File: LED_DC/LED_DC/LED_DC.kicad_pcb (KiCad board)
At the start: 2 copper layers, 98.4 x 98.4 mm, 49 parts, among them J1 Conn_01x04, J2 Display Port GPIO, J3 Conn_01x05, Q1 FDV304P, Q2 FDV304P, Q3 FDV304P, Q4 FDV304P, Q5 FDV304P, Q6 FDV304P, Q7 FDV304P, Q8 FDV304P, SW1 SW_Push_45deg, SW2 SW_Push_45deg, SW3 SW_Push_45deg, SW4 SW_Push_45deg, U1 74HC238, U2 ULN2803A, U3 KCSA02-136, U4 KCSA02-136, U5 KCSA02-136, U6 KCSA02-136, U7 KCSA02-136, U8 KCSA02-136, U9 KCSA02-136

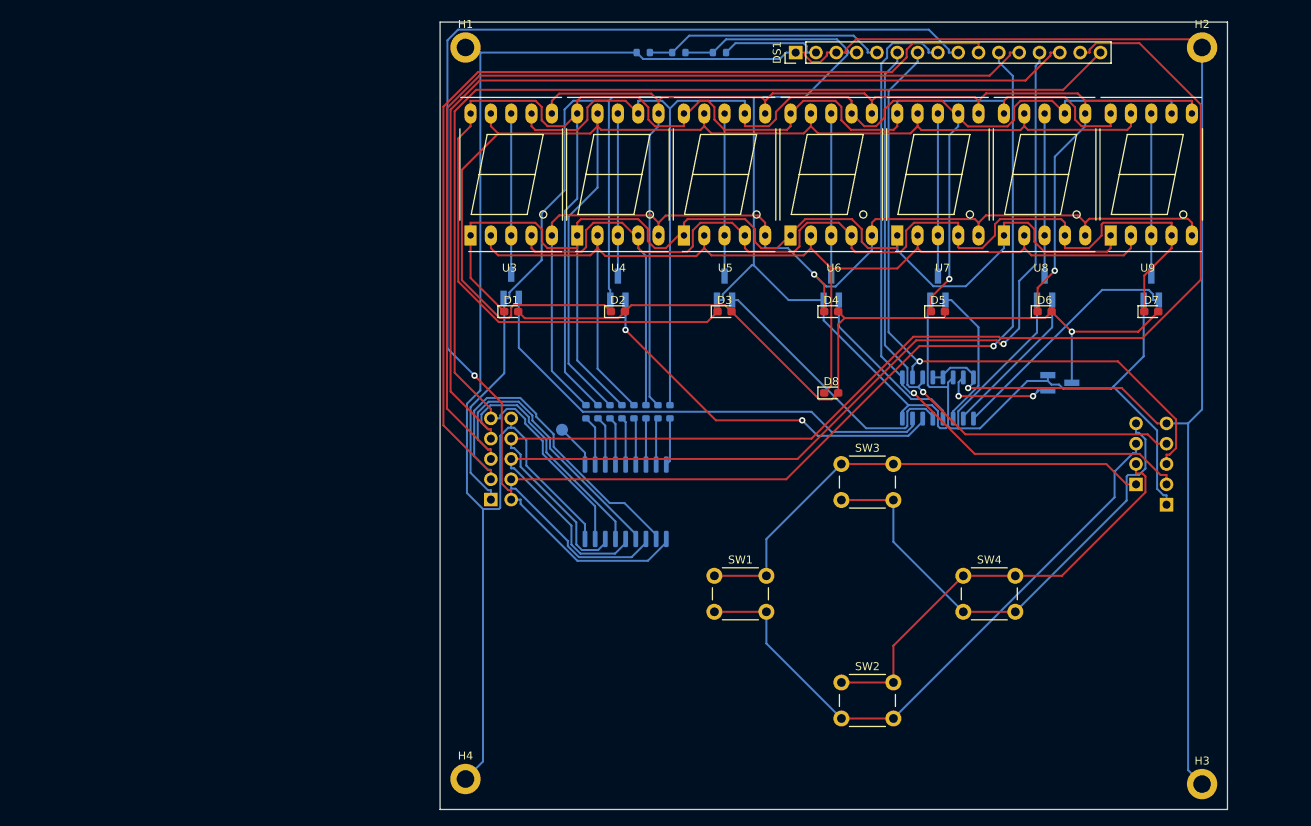
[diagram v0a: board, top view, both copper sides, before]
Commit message: Updated PCB.
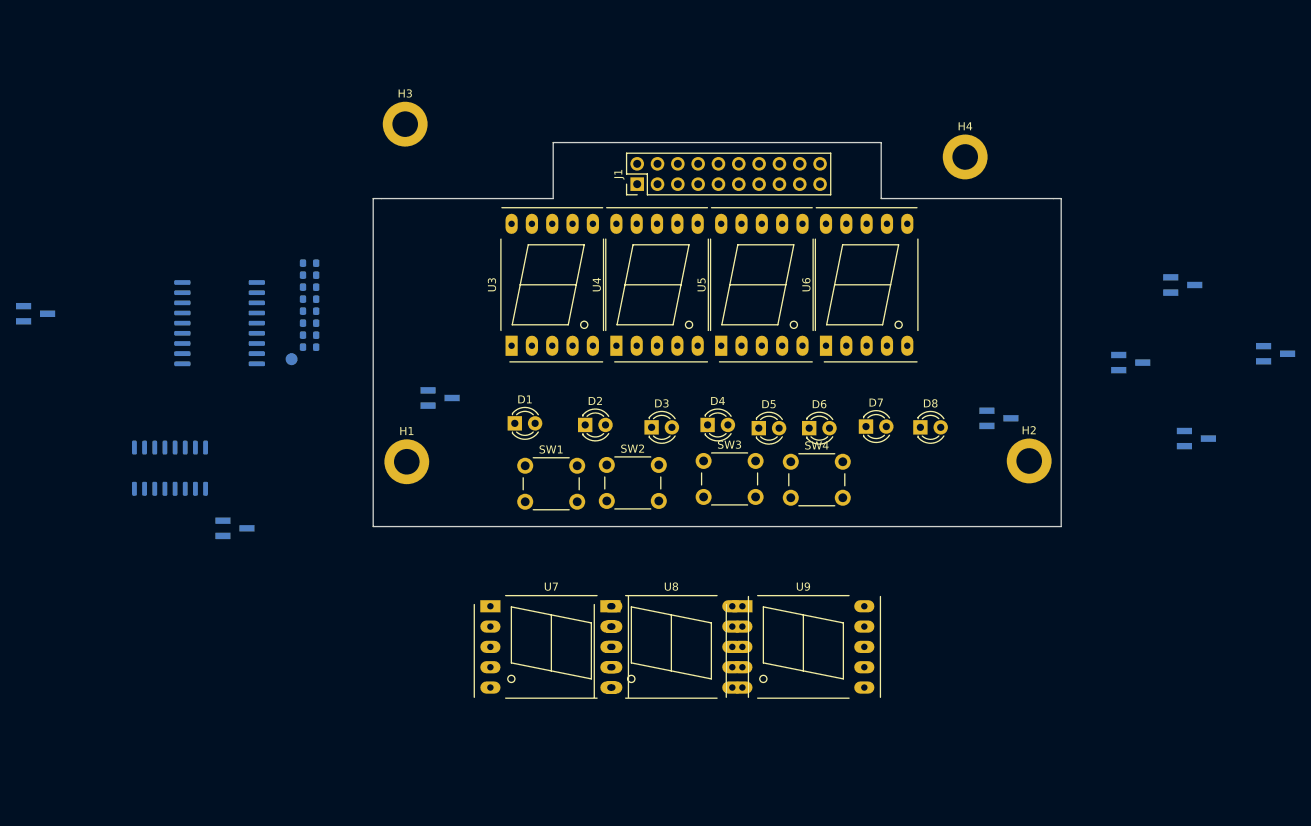
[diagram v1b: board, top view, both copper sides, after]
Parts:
- removed DS1: HY1602E, Connector_PinHeader_2.54mm:PinHeader_1x16_P2.54mm_Vertical
- removed J2: Display Port GPIO, Connector_PinHeader_2.54mm:PinHeader_2x05_P2.54mm_Vertical
- removed J3: Conn_01x05, Connector_PinHeader_2.54mm:PinHeader_1x05_P2.54mm_Vertical
- removed R1, R2, R3: R_Small, Resistor_SMD:R_0603_1608Metric
- D1, D2, D3, D4, D5, D6, D7, D8: footprint LED_SMD:LED_0603_1608Metric_Pad1.05x0.95mm_HandSolder -> LED_THT:LED_D3.0mm
- H1, H2, H3, H4: footprint MountingHole:MountingHole_2.2mm_M2_DIN965_Pad -> MountingHole:MountingHole_3.2mm_M3_DIN965_Pad
- J1: value Conn_01x04 -> MCU interface; footprint Connector_PinHeader_2.54mm:PinHeader_1x04_P2.54mm_Vertical -> Connector_PinHeader_2.54mm:PinHeader_2x10_P2.54mm_Vertical; moved to F.Cu
- moved H3 129.3 mm to (158.2, 53.4)
- moved H4 99.7 mm to (228.2, 57.5)
- moved U1 96.4 mm to (128.8, 96.4)
- moved Q6 80.4 mm to (136.9, 103.9), turned to 0 degrees
- moved J1 72.8 mm to (187.2, 60.9), turned to 90 degrees
- moved Q2 69.4 mm to (267.0, 82.1), turned to 0 degrees
- moved U7 68.8 mm to (168.8, 113.7), turned to 0 degrees
- moved U8 67.6 mm to (183.8, 113.7), turned to 0 degrees
- moved U9 65.3 mm to (200.3, 113.7), turned to 0 degrees
- moved Q1 59.5 mm to (112.0, 77.1), turned to 0 degrees
- moved H2 56.0 mm to (236.2, 95.5)
- moved U2 55.4 mm to (135.0, 78.3), turned to 0 degrees
- moved H1 52.3 mm to (158.4, 95.6)
- moved R4 45.8 mm to (146.2, 81.3), turned to 0 degrees
- moved R5 44.6 mm to (146.2, 79.8), turned to 0 degrees
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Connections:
- J1 pad 1: KEY_ROW1 -> +5V
- J1 pad 2: KEY_ROW2 -> +5V
- J1 pad 3: KEY_COL1 -> D0
- J1 pad 4: KEY_COL2 -> D1
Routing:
- net GND: track 352.0 -> 0.00 mm, vias 1 -> 0
- net +5V: track 301.5 -> 0.00 mm
- net G: track 204.7 -> 0.00 mm
- net F: track 177.0 -> 0.00 mm
- net A: track 167.9 -> 0.00 mm, vias 1 -> 0
- net D1: track 163.0 -> 0.00 mm
- net B: track 158.7 -> 0.00 mm, vias 1 -> 0
- net D6: track 157.0 -> 0.00 mm
- net D3: track 156.5 -> 0.00 mm
- net D5: track 153.2 -> 0.00 mm
- net D0: track 151.0 -> 0.00 mm, vias 1 -> 0
- net E: track 148.4 -> 0.00 mm
- net D7: track 148.2 -> 0.00 mm
- net C: track 145.2 -> 0.00 mm
- net D: track 135.7 -> 0.00 mm
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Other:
- board size 98.4 x 98.4 mm -> 86 x 48 mm
